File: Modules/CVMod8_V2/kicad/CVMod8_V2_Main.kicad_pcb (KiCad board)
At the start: 2 copper layers, 100.8 x 85 mm, 68 parts, among them U1 TL074, U10 79L05, U2 TL074, U3 TL074, U4 TL074, U5 TL074, U6 TL074, U7 TL074, U8 TL074, U9 78L05

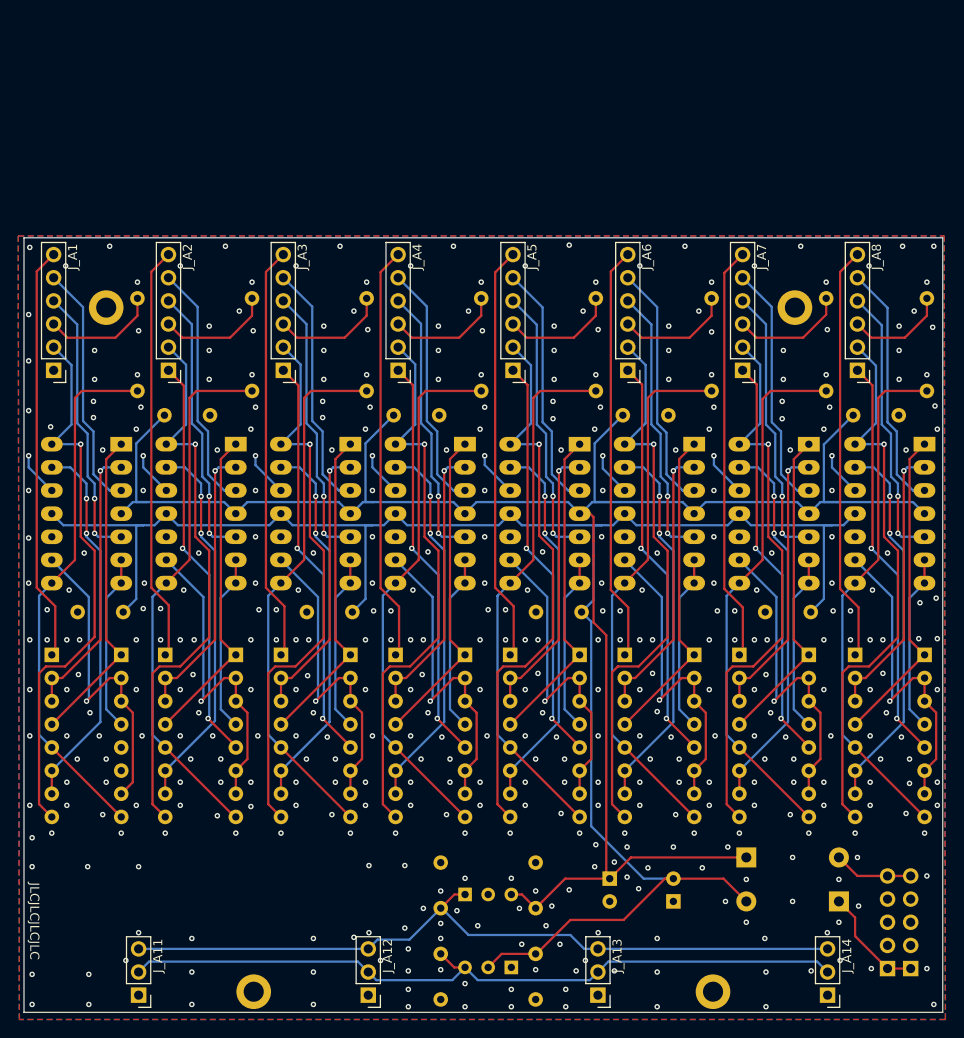
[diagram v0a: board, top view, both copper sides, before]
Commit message: Release SMD CVMod8 V2.
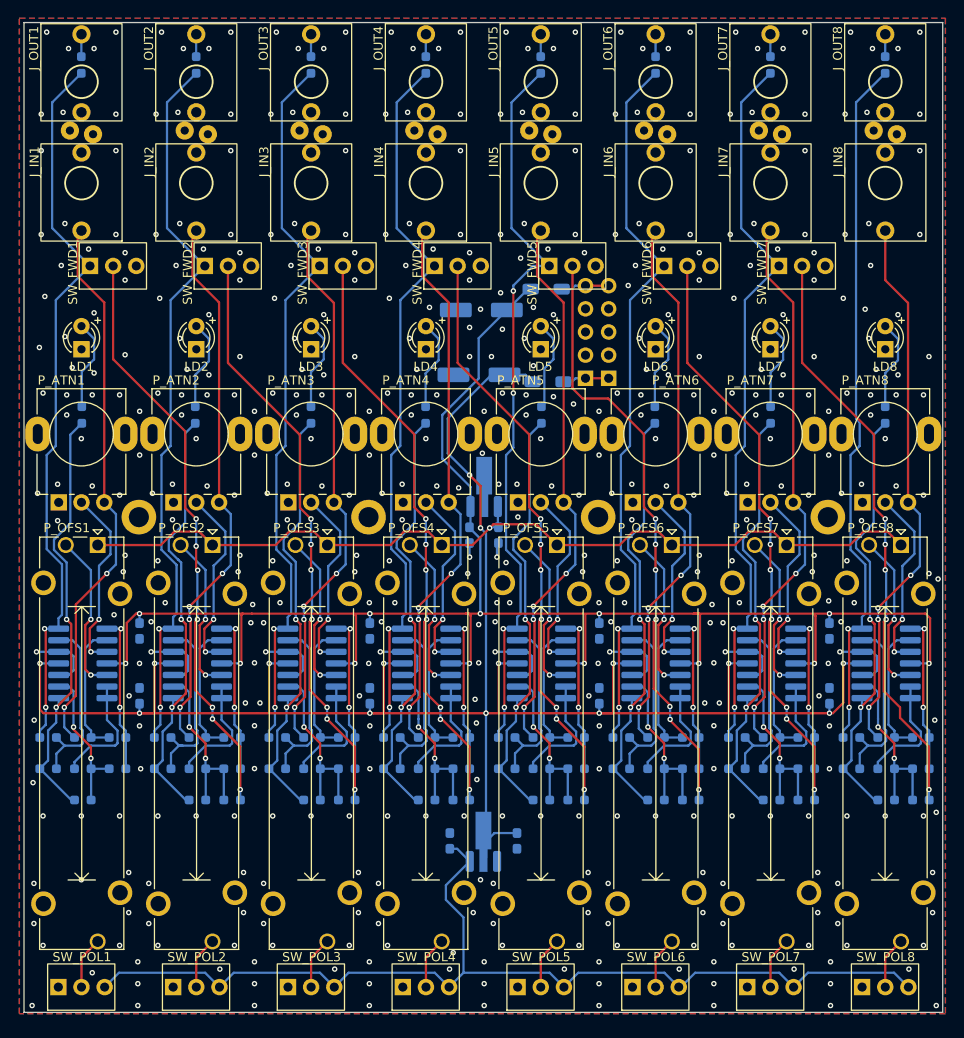
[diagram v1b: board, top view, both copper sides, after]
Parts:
- removed J_A1, J_A2, J_A3, J_A4, J_A5, J_A6, J_A7, J_A8: Conn_01x06_Male, Connector_PinHeader_2.54mm:PinHeader_1x06_P2.54mm_Vertical
- removed J_A11, J_A12, J_A13, J_A14: Conn_01x03_Male, Connector_PinHeader_2.54mm:PinHeader_1x03_P2.54mm_Vertical
- removed the REF** at (116.1, 148.1)
- removed the REF** at (65.7, 148.1)
- removed the REF** at (125.1, 73.0)
- removed the REF** at (49.5, 73.0)
- removed RN1, RN10, RN11, RN12, RN13, RN14, RN15, RN16, RN2, RN3, RN4, RN5, RN6, RN7, RN8, RN9: 100k, Resistor_THT:R_Array_SIP8
- added J_IN1: PJ301M-12, Eurorack:PJ301M-12 Offset, F.Cu at (46.8, 59.4)
- added J_IN2: PJ301M-12, Eurorack:PJ301M-12 Offset, F.Cu at (59.4, 59.4)
- added J_IN3: PJ301M-12, Eurorack:PJ301M-12 Offset, F.Cu at (72.0, 59.4)
- added J_IN4: PJ301M-12, Eurorack:PJ301M-12 Offset, F.Cu at (84.6, 59.4)
- added J_IN5: PJ301M-12, Eurorack:PJ301M-12 Offset, F.Cu at (97.2, 59.4)
- added J_IN6: PJ301M-12, Eurorack:PJ301M-12 Offset, F.Cu at (109.8, 59.4)
- added J_IN7: PJ301M-12, Eurorack:PJ301M-12 Offset, F.Cu at (122.4, 59.4)
- added J_IN8: PJ301M-12, Eurorack:PJ301M-12 Offset, F.Cu at (135.0, 59.4)
- added J_OUT1: PJ301M-12, Eurorack:PJ301M-12 Offset, F.Cu at (46.8, 48.2)
- added J_OUT2: PJ301M-12, Eurorack:PJ301M-12 Offset, F.Cu at (59.4, 48.2)
- added J_OUT3: PJ301M-12, Eurorack:PJ301M-12 Offset, F.Cu at (72.0, 48.2)
- added J_OUT4: PJ301M-12, Eurorack:PJ301M-12 Offset, F.Cu at (84.6, 48.2)
- added J_OUT5: PJ301M-12, Eurorack:PJ301M-12 Offset, F.Cu at (97.2, 48.2)
- added J_OUT6: PJ301M-12, Eurorack:PJ301M-12 Offset, F.Cu at (109.8, 48.2)
- added J_OUT7: PJ301M-12, Eurorack:PJ301M-12 Offset, F.Cu at (122.4, 48.2)
- added J_OUT8: PJ301M-12, Eurorack:PJ301M-12 Offset, F.Cu at (135.0, 48.2)
- added LD1: LED (Bi), LED_THT:LED_D3.0mm_FlatTop, F.Cu at (46.8, 77.6)
- added LD2: LED (Bi), LED_THT:LED_D3.0mm_FlatTop, F.Cu at (59.4, 77.6)
- added LD3: LED (Bi), LED_THT:LED_D3.0mm_FlatTop, F.Cu at (72.0, 77.6)
- added LD4: LED (Bi), LED_THT:LED_D3.0mm_FlatTop, F.Cu at (84.6, 77.6)
- added LD5: LED (Bi), LED_THT:LED_D3.0mm_FlatTop, F.Cu at (97.2, 77.6)
- added LD6: LED (Bi), LED_THT:LED_D3.0mm_FlatTop, F.Cu at (109.8, 77.6)
- added LD7: LED (Bi), LED_THT:LED_D3.0mm_FlatTop, F.Cu at (122.4, 77.6)
- added LD8: LED (Bi), LED_THT:LED_D3.0mm_FlatTop, F.Cu at (135.0, 77.6)
- added P_ATN1: B100k, Eurorack:Potentiometer Song Huei 9mm Trimmer, F.Cu at (46.8, 86.9)
- added P_ATN2: B100k, Eurorack:Potentiometer Song Huei 9mm Trimmer, F.Cu at (59.4, 86.9)
- added P_ATN3: B100k, Eurorack:Potentiometer Song Huei 9mm Trimmer, F.Cu at (72.0, 86.9)
- added P_ATN4: B100k, Eurorack:Potentiometer Song Huei 9mm Trimmer, F.Cu at (84.6, 86.9)
- added P_ATN5: B100k, Eurorack:Potentiometer Song Huei 9mm Trimmer, F.Cu at (97.2, 86.9)
- added P_ATN6: B100k, Eurorack:Potentiometer Song Huei 9mm Trimmer, F.Cu at (109.8, 86.9)
- added P_ATN7: B100k, Eurorack:Potentiometer Song Huei 9mm Trimmer, F.Cu at (122.4, 86.9)
- added P_ATN8: B100k, Eurorack:Potentiometer Song Huei 9mm Trimmer, F.Cu at (135.0, 86.9)
- added P_OFS1: B100k, Potentiometer_THT:Potentiometer_Bourns_PTA3043_Single_Slide, F.Cu at (48.6, 99.1)
- added P_OFS2: B100k, Potentiometer_THT:Potentiometer_Bourns_PTA3043_Single_Slide, F.Cu at (61.2, 99.1)
- added P_OFS3: B100k, Potentiometer_THT:Potentiometer_Bourns_PTA3043_Single_Slide, F.Cu at (73.8, 99.1)
- added P_OFS4: B100k, Potentiometer_THT:Potentiometer_Bourns_PTA3043_Single_Slide, F.Cu at (86.3, 99.1)
- added P_OFS5: B100k, Potentiometer_THT:Potentiometer_Bourns_PTA3043_Single_Slide, F.Cu at (99.0, 99.1)
- added P_OFS6: B100k, Potentiometer_THT:Potentiometer_Bourns_PTA3043_Single_Slide, F.Cu at (111.6, 99.1)
- added P_OFS7: B100k, Potentiometer_THT:Potentiometer_Bourns_PTA3043_Single_Slide, F.Cu at (124.2, 99.1)
- added P_OFS8: B100k, Potentiometer_THT:Potentiometer_Bourns_PTA3043_Single_Slide, F.Cu at (136.7, 99.1)
- added R10: 1k, Resistor_SMD:R_0603_1608Metric_Pad0.98x0.95mm_HandSolder, B.Cu at (59.3, 84.8)
- added R11: 1k, Resistor_SMD:R_0603_1608Metric_Pad0.98x0.95mm_HandSolder, B.Cu at (72.0, 84.8)
- added R12: 1k, Resistor_SMD:R_0603_1608Metric_Pad0.98x0.95mm_HandSolder, B.Cu at (84.6, 84.8)
- added R13: 1k, Resistor_SMD:R_0603_1608Metric_Pad0.98x0.95mm_HandSolder, B.Cu at (97.3, 84.8)
- added R14: 1k, Resistor_SMD:R_0603_1608Metric_Pad0.98x0.95mm_HandSolder, B.Cu at (109.7, 84.8)
- added R15: 1k, Resistor_SMD:R_0603_1608Metric_Pad0.98x0.95mm_HandSolder, B.Cu at (122.4, 84.8)
- added R16: 1k, Resistor_SMD:R_0603_1608Metric_Pad0.98x0.95mm_HandSolder, B.Cu at (135.0, 84.8)
- added R17: 100k, Resistor_SMD:R_0603_1608Metric_Pad0.98x0.95mm_HandSolder, B.Cu at (50.8, 120.2)
- added R18: 100k, Resistor_SMD:R_0603_1608Metric_Pad0.98x0.95mm_HandSolder, B.Cu at (47.0, 120.2)
- added R19: 100k, Resistor_SMD:R_0603_1608Metric_Pad0.98x0.95mm_HandSolder, B.Cu at (43.2, 120.2)
- added R20: 100k, Resistor_SMD:R_0603_1608Metric_Pad0.98x0.95mm_HandSolder, B.Cu at (50.8, 123.6)
- added R21: 100k, Resistor_SMD:R_0603_1608Metric_Pad0.98x0.95mm_HandSolder, B.Cu at (47.0, 123.6)
- added R22: 100k, Resistor_SMD:R_0603_1608Metric_Pad0.98x0.95mm_HandSolder, B.Cu at (43.2, 123.6)
- added R23: 100k, Resistor_SMD:R_0603_1608Metric_Pad0.98x0.95mm_HandSolder, B.Cu at (47.0, 127.0)
- added R24: 100k, Resistor_SMD:R_0603_1608Metric_Pad0.98x0.95mm_HandSolder, B.Cu at (63.3, 120.2)
- added R25: 100k, Resistor_SMD:R_0603_1608Metric_Pad0.98x0.95mm_HandSolder, B.Cu at (59.5, 120.2)
- added R26: 100k, Resistor_SMD:R_0603_1608Metric_Pad0.98x0.95mm_HandSolder, B.Cu at (55.7, 120.2)
- added R27: 100k, Resistor_SMD:R_0603_1608Metric_Pad0.98x0.95mm_HandSolder, B.Cu at (63.3, 123.6)
- added R28: 100k, Resistor_SMD:R_0603_1608Metric_Pad0.98x0.95mm_HandSolder, B.Cu at (59.5, 123.6)
- added R29: 100k, Resistor_SMD:R_0603_1608Metric_Pad0.98x0.95mm_HandSolder, B.Cu at (55.7, 123.6)
- added R30: 100k, Resistor_SMD:R_0603_1608Metric_Pad0.98x0.95mm_HandSolder, B.Cu at (63.3, 127.0)
- added R31: 100k, Resistor_SMD:R_0603_1608Metric_Pad0.98x0.95mm_HandSolder, B.Cu at (59.5, 127.0)
- added R32: 100k, Resistor_SMD:R_0603_1608Metric_Pad0.98x0.95mm_HandSolder, B.Cu at (75.9, 120.2)
- added R33: 100k, Resistor_SMD:R_0603_1608Metric_Pad0.98x0.95mm_HandSolder, B.Cu at (72.1, 120.2)
- added R34: 100k, Resistor_SMD:R_0603_1608Metric_Pad0.98x0.95mm_HandSolder, B.Cu at (68.3, 120.2)
- added R35: 100k, Resistor_SMD:R_0603_1608Metric_Pad0.98x0.95mm_HandSolder, B.Cu at (75.9, 123.6)
- added R36: 100k, Resistor_SMD:R_0603_1608Metric_Pad0.98x0.95mm_HandSolder, B.Cu at (72.1, 123.6)
- added R37: 100k, Resistor_SMD:R_0603_1608Metric_Pad0.98x0.95mm_HandSolder, B.Cu at (68.3, 123.6)
- added R38: 100k, Resistor_SMD:R_0603_1608Metric_Pad0.98x0.95mm_HandSolder, B.Cu at (75.9, 127.0)
- added R39: 100k, Resistor_SMD:R_0603_1608Metric_Pad0.98x0.95mm_HandSolder, B.Cu at (72.1, 127.0)
- added R40: 100k, Resistor_SMD:R_0603_1608Metric_Pad0.98x0.95mm_HandSolder, B.Cu at (88.5, 120.2)
- added R41: 100k, Resistor_SMD:R_0603_1608Metric_Pad0.98x0.95mm_HandSolder, B.Cu at (84.7, 120.2)
- added R42: 100k, Resistor_SMD:R_0603_1608Metric_Pad0.98x0.95mm_HandSolder, B.Cu at (80.9, 120.2)
- added R43: 100k, Resistor_SMD:R_0603_1608Metric_Pad0.98x0.95mm_HandSolder, B.Cu at (88.5, 123.6)
- added R44: 100k, Resistor_SMD:R_0603_1608Metric_Pad0.98x0.95mm_HandSolder, B.Cu at (84.7, 123.6)
- added R45: 100k, Resistor_SMD:R_0603_1608Metric_Pad0.98x0.95mm_HandSolder, B.Cu at (80.9, 123.6)
- added R46: 100k, Resistor_SMD:R_0603_1608Metric_Pad0.98x0.95mm_HandSolder, B.Cu at (88.5, 127.0)
- added R47: 100k, Resistor_SMD:R_0603_1608Metric_Pad0.98x0.95mm_HandSolder, B.Cu at (84.7, 127.0)
- added R48: 100k, Resistor_SMD:R_0603_1608Metric_Pad0.98x0.95mm_HandSolder, B.Cu at (101.1, 120.2)
- added R49: 100k, Resistor_SMD:R_0603_1608Metric_Pad0.98x0.95mm_HandSolder, B.Cu at (97.3, 120.2)
- added R50: 100k, Resistor_SMD:R_0603_1608Metric_Pad0.98x0.95mm_HandSolder, B.Cu at (93.5, 120.2)
- added R51: 100k, Resistor_SMD:R_0603_1608Metric_Pad0.98x0.95mm_HandSolder, B.Cu at (101.1, 123.6)
- added R52: 100k, Resistor_SMD:R_0603_1608Metric_Pad0.98x0.95mm_HandSolder, B.Cu at (97.3, 123.6)
- added R53: 100k, Resistor_SMD:R_0603_1608Metric_Pad0.98x0.95mm_HandSolder, B.Cu at (93.5, 123.6)
- added R54: 100k, Resistor_SMD:R_0603_1608Metric_Pad0.98x0.95mm_HandSolder, B.Cu at (101.1, 127.0)
- added R55: 100k, Resistor_SMD:R_0603_1608Metric_Pad0.98x0.95mm_HandSolder, B.Cu at (97.3, 127.0)
- added R56: 100k, Resistor_SMD:R_0603_1608Metric_Pad0.98x0.95mm_HandSolder, B.Cu at (113.7, 120.2)
- added R57: 100k, Resistor_SMD:R_0603_1608Metric_Pad0.98x0.95mm_HandSolder, B.Cu at (109.9, 120.2)
- added R58: 100k, Resistor_SMD:R_0603_1608Metric_Pad0.98x0.95mm_HandSolder, B.Cu at (106.0, 120.2)
- added R59: 100k, Resistor_SMD:R_0603_1608Metric_Pad0.98x0.95mm_HandSolder, B.Cu at (113.7, 123.6)
- added R60: 100k, Resistor_SMD:R_0603_1608Metric_Pad0.98x0.95mm_HandSolder, B.Cu at (109.9, 123.6)
- added R61: 100k, Resistor_SMD:R_0603_1608Metric_Pad0.98x0.95mm_HandSolder, B.Cu at (106.0, 123.6)
- added R62: 100k, Resistor_SMD:R_0603_1608Metric_Pad0.98x0.95mm_HandSolder, B.Cu at (113.7, 127.0)
- added R63: 100k, Resistor_SMD:R_0603_1608Metric_Pad0.98x0.95mm_HandSolder, B.Cu at (109.9, 127.0)
- added R64: 100k, Resistor_SMD:R_0603_1608Metric_Pad0.98x0.95mm_HandSolder, B.Cu at (126.3, 120.2)
- added R65: 100k, Resistor_SMD:R_0603_1608Metric_Pad0.98x0.95mm_HandSolder, B.Cu at (122.5, 120.2)
- added R66: 100k, Resistor_SMD:R_0603_1608Metric_Pad0.98x0.95mm_HandSolder, B.Cu at (118.7, 120.2)
- added R67: 100k, Resistor_SMD:R_0603_1608Metric_Pad0.98x0.95mm_HandSolder, B.Cu at (126.3, 123.6)
- added R68: 100k, Resistor_SMD:R_0603_1608Metric_Pad0.98x0.95mm_HandSolder, B.Cu at (122.5, 123.6)
- added R69: 100k, Resistor_SMD:R_0603_1608Metric_Pad0.98x0.95mm_HandSolder, B.Cu at (118.7, 123.6)
- added R70: 100k, Resistor_SMD:R_0603_1608Metric_Pad0.98x0.95mm_HandSolder, B.Cu at (126.3, 127.0)
- added R71: 100k, Resistor_SMD:R_0603_1608Metric_Pad0.98x0.95mm_HandSolder, B.Cu at (122.5, 127.0)
- added R72: 100k, Resistor_SMD:R_0603_1608Metric_Pad0.98x0.95mm_HandSolder, B.Cu at (138.9, 120.2)
- added R73: 100k, Resistor_SMD:R_0603_1608Metric_Pad0.98x0.95mm_HandSolder, B.Cu at (135.1, 120.2)
- added R74: 100k, Resistor_SMD:R_0603_1608Metric_Pad0.98x0.95mm_HandSolder, B.Cu at (131.3, 120.2)
- added R75: 100k, Resistor_SMD:R_0603_1608Metric_Pad0.98x0.95mm_HandSolder, B.Cu at (138.9, 123.6)
- added R76: 100k, Resistor_SMD:R_0603_1608Metric_Pad0.98x0.95mm_HandSolder, B.Cu at (135.1, 123.6)
- added R77: 100k, Resistor_SMD:R_0603_1608Metric_Pad0.98x0.95mm_HandSolder, B.Cu at (131.3, 123.6)
- added R78: 100k, Resistor_SMD:R_0603_1608Metric_Pad0.98x0.95mm_HandSolder, B.Cu at (138.9, 127.0)
- added R79: 100k, Resistor_SMD:R_0603_1608Metric_Pad0.98x0.95mm_HandSolder, B.Cu at (135.1, 127.0)
- added R9: 1k, Resistor_SMD:R_0603_1608Metric_Pad0.98x0.95mm_HandSolder, B.Cu at (46.9, 84.8)
- added REF**: M2 Screw Hole, Eurorack:M2 Screw Hole, F.Cu at (128.7, 96.0)
- added REF**: M2 Screw Hole, Eurorack:M2 Screw Hole, F.Cu at (103.5, 96.0)
- added REF**: M2 Screw Hole, Eurorack:M2 Screw Hole, F.Cu at (53.1, 96.0)
- added REF**: M2 Screw Hole, Eurorack:M2 Screw Hole, F.Cu at (78.3, 96.0)
- added SW_FWD1: SW_SPDT, Eurorack:SPDT, F.Cu at (50.3, 68.5)
- added SW_FWD2: SW_SPDT, Eurorack:SPDT, F.Cu at (62.9, 68.5)
- added SW_FWD3: SW_SPDT, Eurorack:SPDT, F.Cu at (75.5, 68.5)
- added SW_FWD4: SW_SPDT, Eurorack:SPDT, F.Cu at (88.1, 68.5)
- added SW_FWD5: SW_SPDT, Eurorack:SPDT, F.Cu at (100.7, 68.5)
- added SW_FWD6: SW_SPDT, Eurorack:SPDT, F.Cu at (113.3, 68.5)
- added SW_FWD7: SW_SPDT, Eurorack:SPDT, F.Cu at (125.9, 68.5)
- added SW_POL1: SW_SPDT, Eurorack:SPDT, F.Cu at (46.8, 147.6)
- added SW_POL2: SW_SPDT, Eurorack:SPDT, F.Cu at (59.4, 147.6)
- added SW_POL3: SW_SPDT, Eurorack:SPDT, F.Cu at (72.0, 147.6)
- added SW_POL4: SW_SPDT, Eurorack:SPDT, F.Cu at (84.6, 147.6)
- added SW_POL5: SW_SPDT, Eurorack:SPDT, F.Cu at (97.2, 147.6)
- added SW_POL6: SW_SPDT, Eurorack:SPDT, F.Cu at (109.8, 147.6)
- added SW_POL7: SW_SPDT, Eurorack:SPDT, F.Cu at (122.4, 147.6)
- added SW_POL8: SW_SPDT, Eurorack:SPDT, F.Cu at (135.0, 147.6)
- C1, C2: footprint Capacitor_THT:CP_Radial_D6.3mm_P2.50mm -> Capacitor_SMD:CP_Elec_6.3x5.3
- C10, C11, C12, C13, C14, C3, C4, C5, C6, C7, C8, C9: footprint Capacitor_THT:C_Disc_D7.0mm_W2.5mm_P5.00mm -> Capacitor_SMD:C_0603_1608Metric_Pad1.08x0.95mm_HandSolder
- D1, D2: value 1N4001 -> FM4001; footprint Diode_THT:D_DO-41_SOD81_P10.16mm_Horizontal -> Eurorack:D_SOD-123F_AH
- R1, R2, R3, R4, R5, R6, R7, R8: footprint Resistor_THT:R_Axial_DIN0207_L6.3mm_D2.5mm_P10.16mm_Horizontal -> Resistor_SMD:R_0603_1608Metric_Pad0.98x0.95mm_HandSolder
- U1, U2, U3, U4, U5, U6, U7, U8: footprint Package_DIP:DIP-14_W7.62mm_Socket_LongPads -> Eurorack:SO-14_3.9x8.65mm_P1.27mm_AH
- U10, U9: footprint Package_TO_SOT_THT:TO-92_Inline_Wide -> Package_TO_SOT_SMD:SOT-89-3_Handsoldering
- moved PWR1 72.7 mm to (104.7, 75.7)
- moved D1 66.1 mm to (97.8, 71.0)
- moved C10 65.7 mm to (78.5, 115.6), turned to 90 degrees
- moved D2 65.3 mm to (98.0, 81.2)
- moved C1 64.0 mm to (90.7, 73.3), turned to 180 degrees
- moved C2 61.6 mm to (90.4, 80.4), turned to 0 degrees
- moved C11 52.3 mm to (103.6, 108.5), turned to 90 degrees
- moved C4 51.1 mm to (92.6, 98.0), turned to -90 degrees
- moved U9 45.1 mm to (91.0, 92.4), turned to 90 degrees
- moved C8 45.0 mm to (53.2, 115.6), turned to 90 degrees
- moved C3 41.6 mm to (89.4, 98.0), turned to -90 degrees
- moved C9 40.4 mm to (78.5, 108.5), turned to 90 degrees
- moved R1 36.3 mm to (46.8, 46.4)
- moved R6 36.3 mm to (109.8, 46.4)
- moved R2 36.3 mm to (59.4, 46.4)
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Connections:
- C10 pad 1: GND -> -12V
- C10 pad 2: +12V -> GND
- C11 pad 1: -12V -> GND
- C11 pad 2: GND -> +12V
- C13 pad 1: -12V -> GND
- C13 pad 2: GND -> +12V
- C4 pad 1: GND -> +5V
- C4 pad 2: -12V -> GND
- C5 pad 1: +5V -> GND
- C5 pad 2: GND -> -12V
- C8 pad 1: GND -> -12V
- C8 pad 2: +12V -> GND
- R1 pad 1: Net-(RN1C-R3.1) -> /OUT1
- R1 pad 2: /LED1 -> Net-(J_OUT1-PadSIG)
- R2 pad 1: Net-(RN3C-R3.1) -> /OUT2
- R2 pad 2: /LED2 -> Net-(J_OUT2-PadSIG)
- R3 pad 1: Net-(RN5C-R3.1) -> /OUT3
- R3 pad 2: /LED3 -> Net-(J_OUT3-PadSIG)
- R4 pad 1: Net-(RN7C-R3.1) -> /OUT4
- R4 pad 2: /LED4 -> Net-(J_OUT4-PadSIG)
- R5 pad 1: Net-(RN10D-R4.2) -> /OUT5
- R5 pad 2: /LED5 -> Net-(J_OUT5-PadSIG)
- R6 pad 1: Net-(RN11C-R3.1) -> /OUT6
- R6 pad 2: /LED6 -> Net-(J_OUT6-PadSIG)
- R7 pad 1: Net-(RN13C-R3.1) -> /OUT7
- R7 pad 2: /LED7 -> Net-(J_OUT7-PadSIG)
- R8 pad 1: Net-(RN15C-R3.1) -> /OUT8
- R8 pad 2: /LED8 -> Net-(J_OUT8-PadSIG)
- U1 pad 8: Net-(RN1C-R3.1) -> Net-(R22-Pad1)
- U2 pad 8: Net-(RN3C-R3.1) -> Net-(R10-Pad1)
- U3 pad 8: Net-(RN5C-R3.1) -> Net-(R11-Pad1)
- U4 pad 8: Net-(RN7C-R3.1) -> Net-(R12-Pad1)
- U5 pad 8: Net-(RN10D-R4.2) -> Net-(R13-Pad1)
- U6 pad 8: Net-(RN11C-R3.1) -> Net-(R14-Pad1)
- U7 pad 8: Net-(RN13C-R3.1) -> Net-(R15-Pad1)
- U8 pad 8: Net-(RN15C-R3.1) -> Net-(R16-Pad1)
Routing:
- net /FWD5: track 0.00 -> 66.3 mm, vias 0 -> 7
- net /FWD3: track 0.00 -> 64.7 mm, vias 0 -> 7
- net /FWD1: track 0.00 -> 64.6 mm, vias 0 -> 7
- net /FWD6: track 0.00 -> 64.6 mm, vias 0 -> 7
- net /FWD2: track 0.00 -> 64.6 mm, vias 0 -> 7
- net /FWD7: track 0.00 -> 64.6 mm, vias 0 -> 5
- net /FWD4: track 0.00 -> 64.6 mm, vias 0 -> 7
- net Net-(J_IN6-PadSIG): track 0.00 -> 60.4 mm, vias 0 -> 4
- net Net-(J_IN7-PadSIG): track 0.00 -> 60.4 mm, vias 0 -> 4
- net Net-(J_IN3-PadSIG): track 0.00 -> 60.4 mm, vias 0 -> 4
- net Net-(J_IN5-PadSIG): track 0.00 -> 60.4 mm, vias 0 -> 4
- net Net-(J_IN4-PadSIG): track 0.00 -> 60.4 mm, vias 0 -> 4
- net Net-(J_IN2-PadSIG): track 0.00 -> 60.4 mm, vias 0 -> 4
- net Net-(J_IN1-PadSIG): track 0.00 -> 60.3 mm, vias 0 -> 2
- net Net-(J_IN8-PadSIG): track 0.00 -> 60.1 mm, vias 0 -> 4
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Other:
- board size 100.8 x 85 mm -> 100.8 x 108.6 mm
- board text added: "CVMod8 V2 v2.2"
- board text removed: "CVMod8 V2 v2.1"
